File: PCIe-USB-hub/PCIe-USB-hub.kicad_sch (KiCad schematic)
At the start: 17 parts, among them J1 PCIexpress_x1, J2 USB3_A_Stacked, J3 USB3_A_Stacked, J4 USB3_A_Stacked, J5 USB3_A_Stacked, J6 USB3_A_Stacked, J7 Barrel_Jack_MountingPin

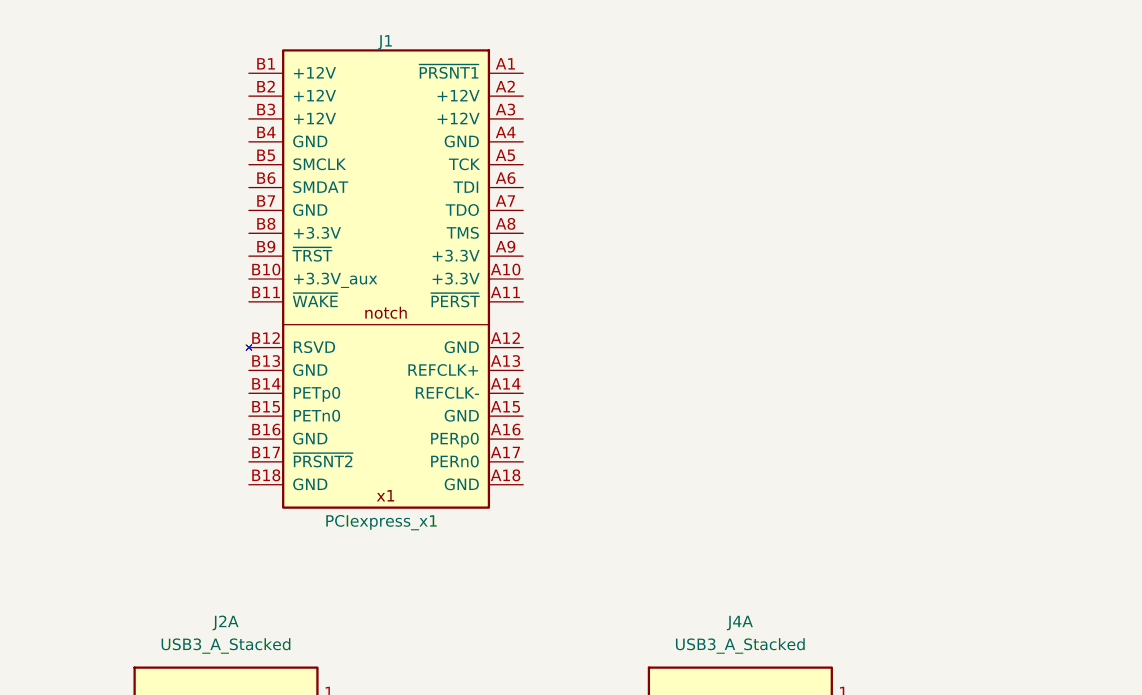
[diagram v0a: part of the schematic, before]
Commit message: Чут изменений
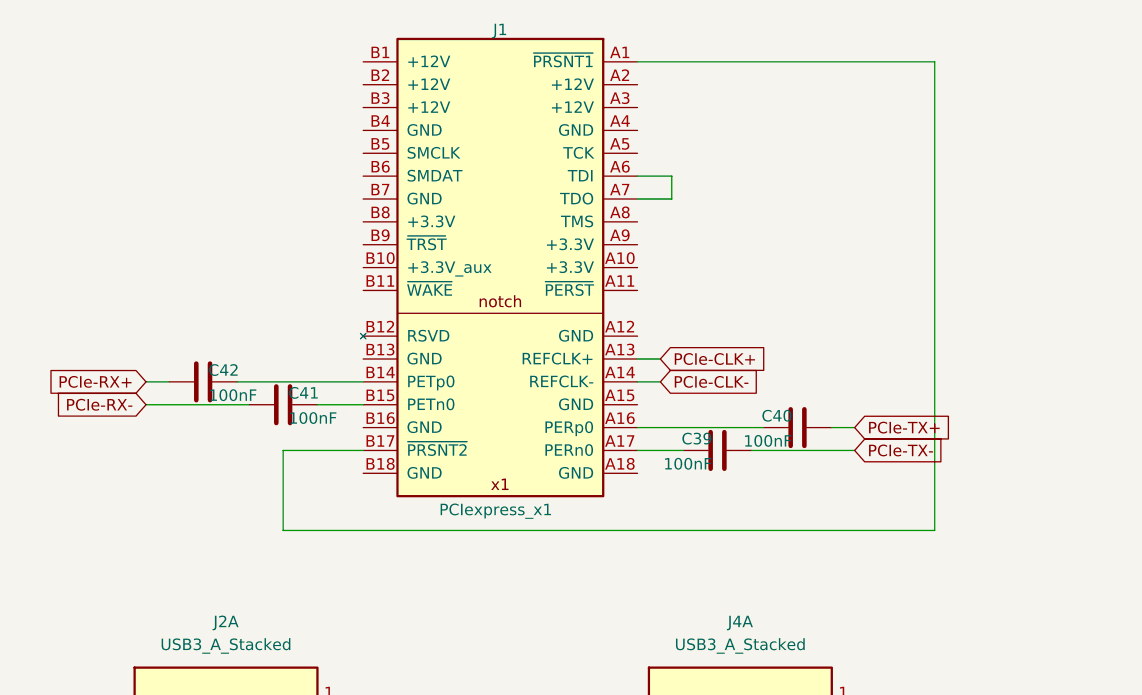
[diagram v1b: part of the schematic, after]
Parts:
- added C39, C40, C41, C42: 100nF, Capacitor_SMD:C_0402_1005Metric, symbol Device:C
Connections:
- net at J1.A1 (~{PRSNT1}): now also J1.B17 (~{PRSNT2})
- net PCIe-CLK+: now reaches J1.A13 (REFCLK+)
- net PCIe-CLK-: now reaches J1.A14 (REFCLK-)
- net at J1.A16 (PERp0): now also C40.2
- net at J1.A17 (PERn0): now also C39.2
- net at J1.A6 (TDI): now also J1.A7 (TDO)
- net at J1.B14 (PETp0): now also C42.2
- net at J1.B15 (PETn0): now also C41.2
- new net PCIe-RX+: C42.1
- new net PCIe-RX-: C41.1
- new net PCIe-TX+: C40.1
- new net PCIe-TX-: C39.1
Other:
- moved on the sheet: J1
